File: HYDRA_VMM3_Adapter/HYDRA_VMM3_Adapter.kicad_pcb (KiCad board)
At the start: 8 copper layers, 121.5 x 31.5 mm, 7 parts, among them J1 ME1014010101011, J2 ME1014010101011, J3 ME1014010101011, J4 ME1014010101011, J5 ME1014010101011, J6 ME1014010101011

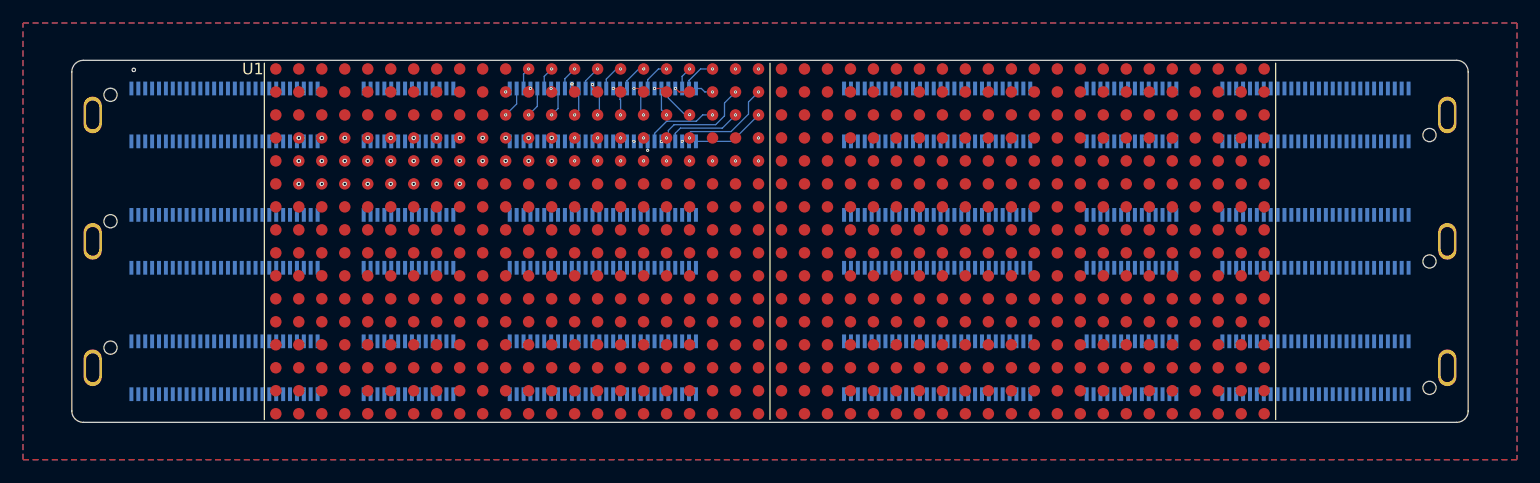
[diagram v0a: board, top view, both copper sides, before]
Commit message: .
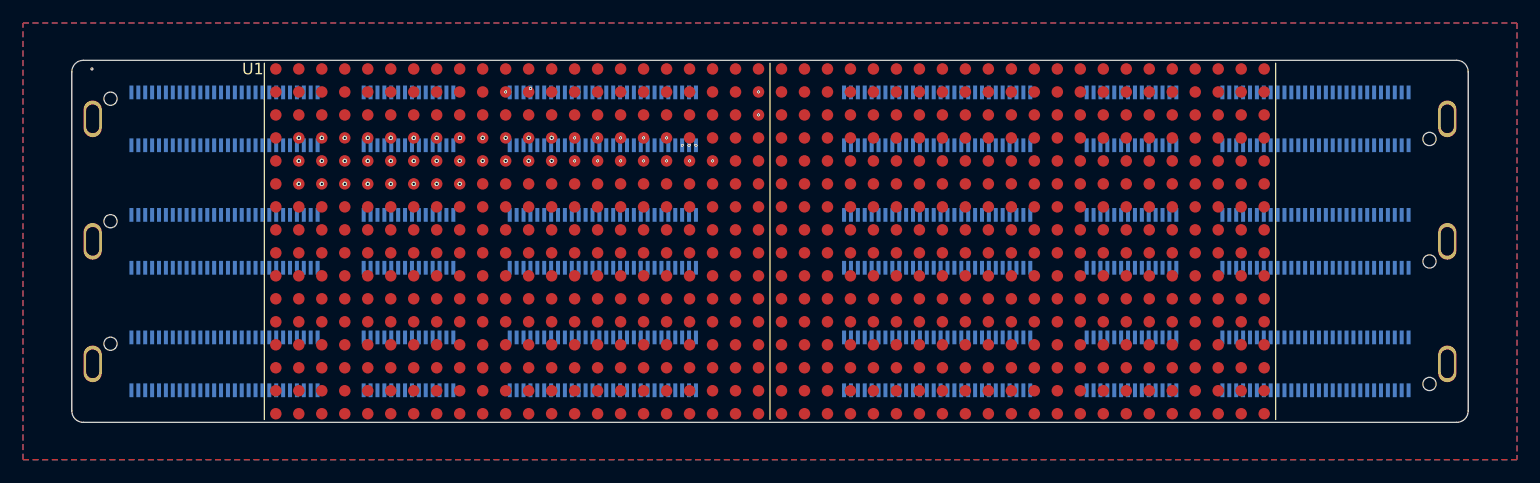
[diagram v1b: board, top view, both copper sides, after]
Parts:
- moved J1 0.34 mm to (137.7, 55.6)
- moved J4 0.34 mm to (75.7, 55.6)
- moved J3 0.34 mm to (137.7, 76.9)
- moved J6 0.34 mm to (75.7, 76.9)
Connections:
- J4 pad A36: Col_9-Row_4 -> Col_9-Row_5
- J4 pad A37: Col_9-Row_5 -> Col_9-Row_4
- J4 pad A38: Col_10-Row_4 -> Col_10-Row_5
- J4 pad A39: Col_10-Row_5 -> Col_10-Row_4
- J4 pad A40: Col_11-Row_4 -> Col_11-Row_5
- J4 pad A41: Col_11-Row_5 -> Col_11-Row_4
- J4 pad A42: Col_12-Row_4 -> Col_12-Row_5
- J4 pad A43: Col_12-Row_5 -> Col_12-Row_4
- J4 pad A44: Col_13-Row_4 -> Col_13-Row_5
- J4 pad A45: Col_13-Row_5 -> Col_13-Row_4
- J4 pad A46: Col_14-Row_4 -> Col_14-Row_5
- J4 pad A47: Col_14-Row_5 -> Col_14-Row_4
- J4 pad A48: Col_15-Row_4 -> Col_15-Row_5
- J4 pad A49: Col_15-Row_5 -> Col_15-Row_4
- J4 pad A50: Col_16-Row_4 -> Col_16-Row_5
- J4 pad A51: Col_16-Row_5 -> Col_16-Row_4
- J4 pad A52: Col_17-Row_4 -> Col_17-Row_5
- J4 pad A53: Col_17-Row_5 -> Col_17-Row_4
- J4 pad A54: Col_18-Row_4 -> Col_18-Row_5
- J4 pad A55: Col_18-Row_5 -> Col_18-Row_4
- J4 pad A56: Col_19-Row_4 -> Col_19-Row_5
- J4 pad A57: Col_19-Row_5 -> Col_19-Row_4
- J4 pad A58: Col_20-Row_4 -> Col_20-Row_5
- J4 pad A59: Col_20-Row_5 -> Col_20-Row_4
- J4 pad A60: Col_21-Row_4 -> Col_20-Row_3
- J4 pad A62: Col_22-Row_4 -> Col_21-Row_4
- J4 pad A63: Col_22-Row_5 -> Col_21-Row_1
- J4 pad A64: Col_20-Row_3 -> Col_21-Row_2
- J4 pad A65: Col_21-Row_1 -> Col_21-Row_3
- J4 pad A66: Col_21-Row_2 -> Col_22-Row_5
- J4 pad A67: Col_21-Row_3 -> Col_22-Row_4
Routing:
- net Col_22-Row_5: track 11.1 -> 0.00 mm, vias 2 -> 0
- net Col_22-Row_4: track 10.7 -> 0.00 mm, vias 2 -> 0
- net Col_21-Row_5: track 9.84 -> 0.00 mm, vias 2 -> 0
- net Col_22-Row_1: track 9.62 -> 0.00 mm, vias 2 -> 1
- net Col_21-Row_1: track 9.54 -> 0.00 mm, vias 2 -> 0
- net Col_21-Row_2: track 8.86 -> 0.02 mm, vias 1 -> 0
- net Col_21-Row_3: track 6.61 -> 0.00 mm, vias 1 -> 0
- net Col_20-Row_3: track 6.40 -> 0.00 mm, vias 1 -> 0
- net Col_19-Row_1: track 3.31 -> 0.00 mm, vias 1 -> 0
- net Col_20-Row_1: track 3.16 -> 0.00 mm, vias 1 -> 0
- net Col_18-Row_1: track 2.80 -> 0.00 mm, vias 1 -> 0
- net Col_11-Row_3: track 2.70 -> 0.00 mm, vias 1 -> 0
- net Col_12-Row_3: track 2.61 -> 0.00 mm, vias 1 -> 0
- net Col_17-Row_1: track 2.58 -> 0.00 mm, vias 1 -> 0
- net Col_13-Row_3: track 2.53 -> 0.00 mm, vias 1 -> 0
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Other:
- copper layers 8 -> 10
